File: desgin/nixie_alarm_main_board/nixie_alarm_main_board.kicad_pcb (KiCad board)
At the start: 2 copper layers, 138.3 x 52.9 mm, 114 parts, among them IC1 LM3488MM, IC2 HV5530PG-G, IC3 TPS563219ADDFR, IC4 HV5530PG-G, IC6 CD40109BQNSRQ1, IC7 AP7363-33D-13, IC8 MCP4018T-502E_LT, J1 PJ-094H-SMT-TR, J2 JST XH 2.54 3 pin, J3 USB_C_Receptacle_USB2.0_16P, J5 Goldpin 3pin, Q1 SSM3K35AMFV,L3F, Q2 DMN60H080DS-13, Q3 DMN60H080DS-13, Q4 DMN60H080DS-13, Q5 DMN60H080DS-13, Q6 DMN60H080DS-13, Q7 DMN60H080DS-13, Q8 TPH5200FNH,L1Q, U1 ESP32-S3-WROOM-1

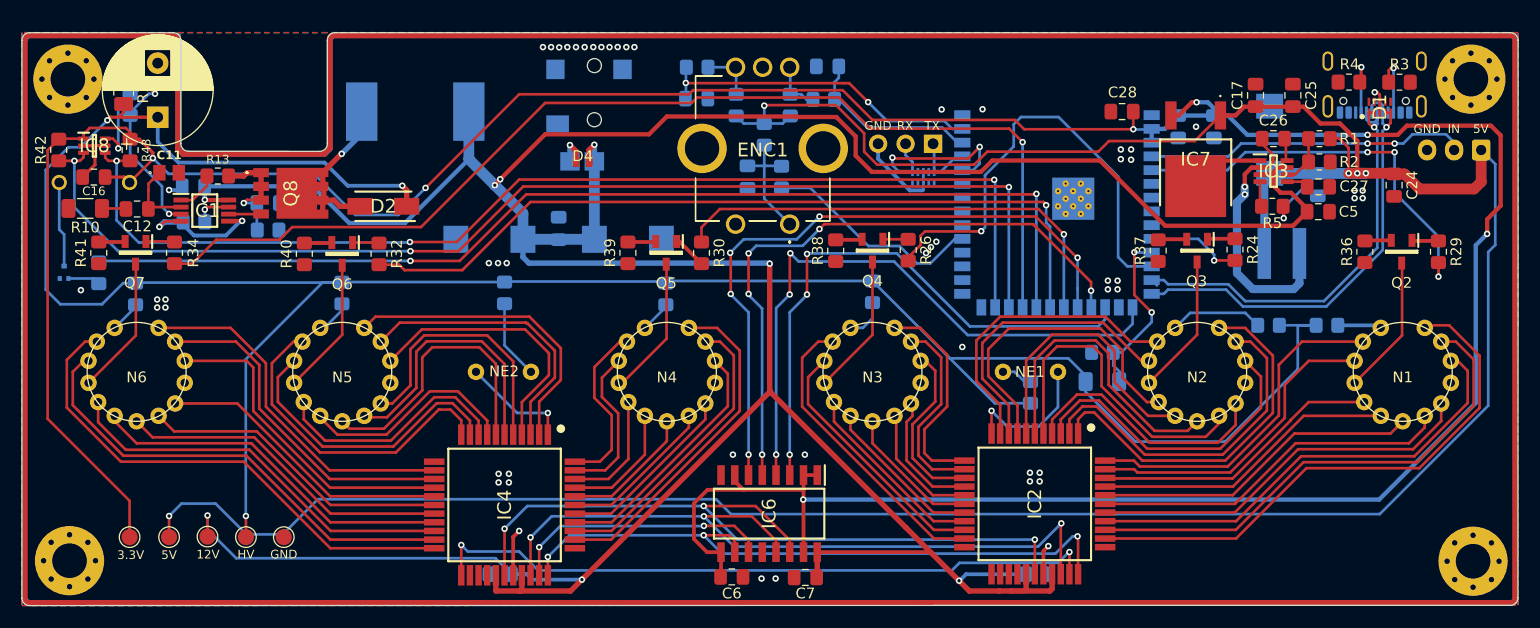
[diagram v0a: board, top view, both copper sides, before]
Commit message: fixes added
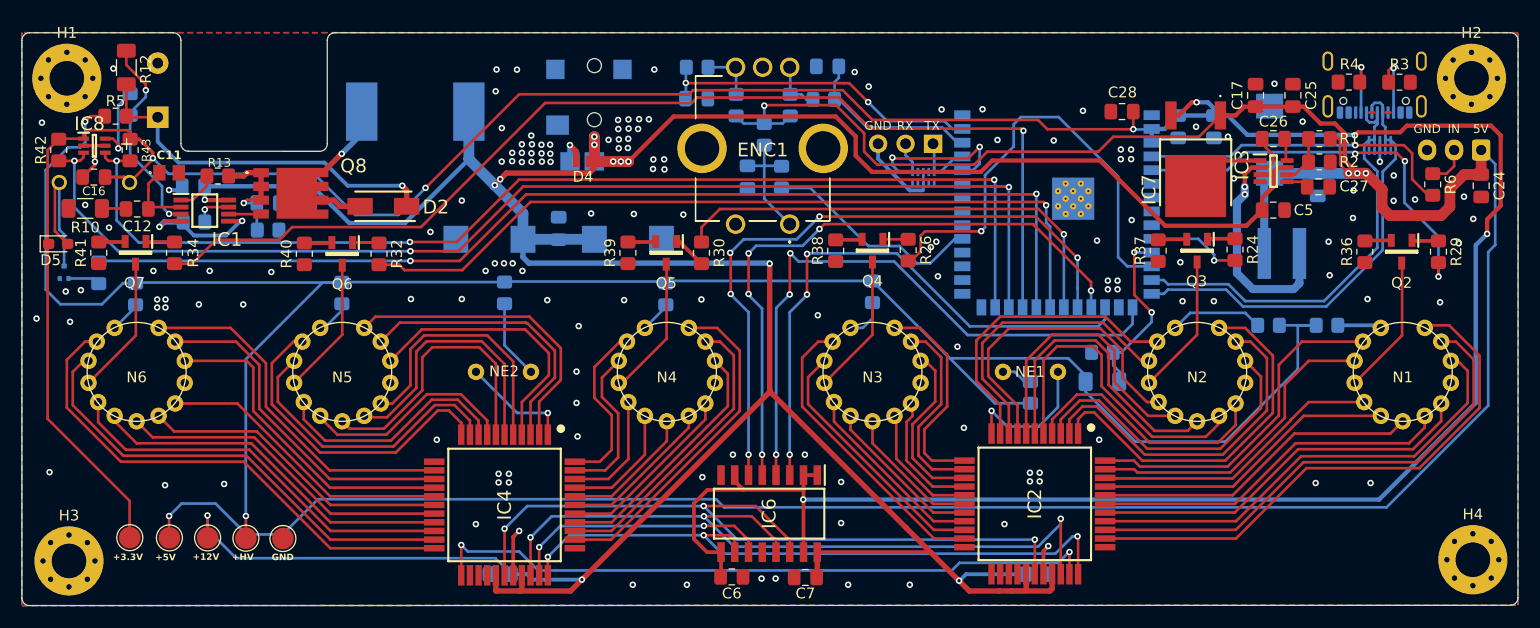
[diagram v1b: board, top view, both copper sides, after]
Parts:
- removed 12V, 3.3V, 5V, HV: TestPoint_Pad_D1.5mm, TestPoint:TestPoint_Pad_D1.5mm
- removed the GND at (111.0, 120.2)
- removed REF** (x4): MountingHole_3.2mm_M3_Pad_Via, MountingHole:MountingHole_3.2mm_M3_Pad_Via
- added +12V: +12V, TestPoint:TestPoint_Pad_D2.0mm, F.Cu at (104.0, 120.3)
- added +3.3V: +3.3V, TestPoint:TestPoint_Pad_D2.0mm, F.Cu at (96.8, 120.2)
- added +5V: +5V, TestPoint:TestPoint_Pad_D2.0mm, F.Cu at (100.5, 120.3)
- added +HV: +HV, TestPoint:TestPoint_Pad_D2.0mm, F.Cu at (107.5, 120.3)
- added D5: CDBUR0520, Diode_SMD:D_0603_1608Metric_Pad1.05x0.95mm_HandSolder, F.Cu at (90.2, 93.1)
- added GND: GND, TestPoint:TestPoint_Pad_D2.0mm, F.Cu at (111.0, 120.3)
- added H1: MountingHole_Pad, MountingHole:MountingHole_3.2mm_M3_Pad_Via, F.Cu at (91.0, 77.8)
- added H2: MountingHole_Pad, MountingHole:MountingHole_3.2mm_M3_Pad_Via, F.Cu at (220.8, 77.8)
- added H3: MountingHole_Pad, MountingHole:MountingHole_3.2mm_M3_Pad_Via, F.Cu at (91.2, 122.4)
- added H4: MountingHole_Pad, MountingHole:MountingHole_3.2mm_M3_Pad_Via, F.Cu at (220.9, 122.3)
- added R6: 470Ω, Resistor_SMD:R_0805_2012Metric_Pad1.20x1.40mm_HandSolder, F.Cu at (217.2, 87.6)
- D1: moved to B.Cu
- J5: value Goldpin 3pin -> Goldpin 3pin
- R5: value 100kΩ -> 0Ω
- moved R5 107.2 mm to (95.5, 81.3), turned to 180 degrees
- moved C24 8.05 mm to (221.7, 87.7)
- moved C5 4.16 mm to (202.5, 90.0)
- moved D1 3.53 mm to (212.3, 84.0), turned to -90 degrees
- moved R12 1.85 mm to (96.5, 76.8)
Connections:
- C2 pad 1: HV -> Net-(D2-K)
- ENC1 pad MH1: (no net) -> GND
- ENC1 pad MH2: (no net) -> GND
- J1 pad MP1: unconnected-(J1-PadMP1) -> GND
- J1 pad MP2: unconnected-(J1-PadMP2) -> GND
- J2 pad 2: LED_DATA -> Net-(J2-Pin_2)
- LS1 pad 2: Net-(LS1--) -> Net-(D5-A)
- R12 pad 1: HV -> Net-(D2-K)
- R36 pad 1: GND -> Net-(Q2-D)
- R36 pad 2: Net-(Q2-S) -> Net-(N1-Padic)
- R37 pad 1: GND -> Net-(Q3-D)
- R37 pad 2: Net-(Q3-S) -> Net-(N2-Padic)
- R38 pad 1: GND -> Net-(Q4-D)
- R38 pad 2: Net-(Q4-S) -> Net-(N3-Padic)
- R39 pad 1: GND -> Net-(Q5-D)
- R39 pad 2: Net-(Q5-S) -> Net-(N4-Padic)
- R40 pad 1: GND -> Net-(Q6-D)
- R40 pad 2: Net-(Q6-S) -> Net-(N5-Padic)
- R41 pad 1: GND -> Net-(Q7-D)
- R41 pad 2: Net-(Q7-S) -> Net-(N6-Padic)
- R5 pad 1: Net-(IC3-PG) -> Net-(D2-K)
- R5 pad 2: +5V -> HV
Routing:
- net (no net): track 801.8 -> 0.00 mm
- net +12V: track 327.3 -> 315.9 mm, vias 8 -> 12
- net HV: track 229.7 -> 222.6 mm
- net Net-(D5-A): track 0.00 -> 6.32 mm
- net Net-(D2-K): track 0.00 -> 5.67 mm
- net Net-(J2-Pin_2): track 0.00 -> 4.28 mm
- net Net-(D2-A): track 15.0 -> 11.0 mm
- net +5V: track 273.4 -> 269.6 mm, vias 6 -> 5
- net Net-(IC3-PG): track 1.98 -> 0.00 mm
- net USB_D-: track 42.4 -> 41.1 mm, vias 1 -> 0
- net Net-(IC2-~{LE}): track 68.8 -> 69.6 mm
- net NX_DOT_6: track 101.7 -> 102.4 mm
- net USB_D+: track 42.4 -> 41.9 mm, vias 1 -> 0
- net GND: track 49.6 -> 49.4 mm, vias 58 -> 152
- net LED_DATA: track 29.9 -> 29.7 mm, vias 2 -> 1
